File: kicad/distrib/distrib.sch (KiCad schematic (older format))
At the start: 35 parts, among them J1 Conn_01x03_Male, J10 Conn_01x03_Male, J11 Conn_01x03_Male, J12 Conn_01x03_Male, J13 Conn_01x03_Male, J14 Conn_01x03_Male, J15 Conn_01x03_Male, J16 Conn_01x03_Male, J17 Conn_01x03_Male, J18 Conn_01x03_Male, J19 Conn_01x03_Male, J2 Conn_01x03_Male, J20 Conn_01x03_Male, J21 Conn_01x03_Male, J22 Conn_01x03_Male, J23 Conn_01x03_Male, J24 Conn_01x03_Male, J25 Conn_01x03_Male, J26 Conn_01x03_Male, J27 Conn_01x03_Male, J28 Conn_01x03_Male, J29 Conn_01x03_Male, J3 Conn_01x03_Male, J30 Conn_01x03_Male, J31 Screw_Terminal_01x02, J4 Conn_01x03_Male, J5 Conn_01x03_Male, J6 Conn_01x03_Male, J7 Conn_01x03_Male, J8 Conn_01x03_Male, J9 Conn_01x03_Male

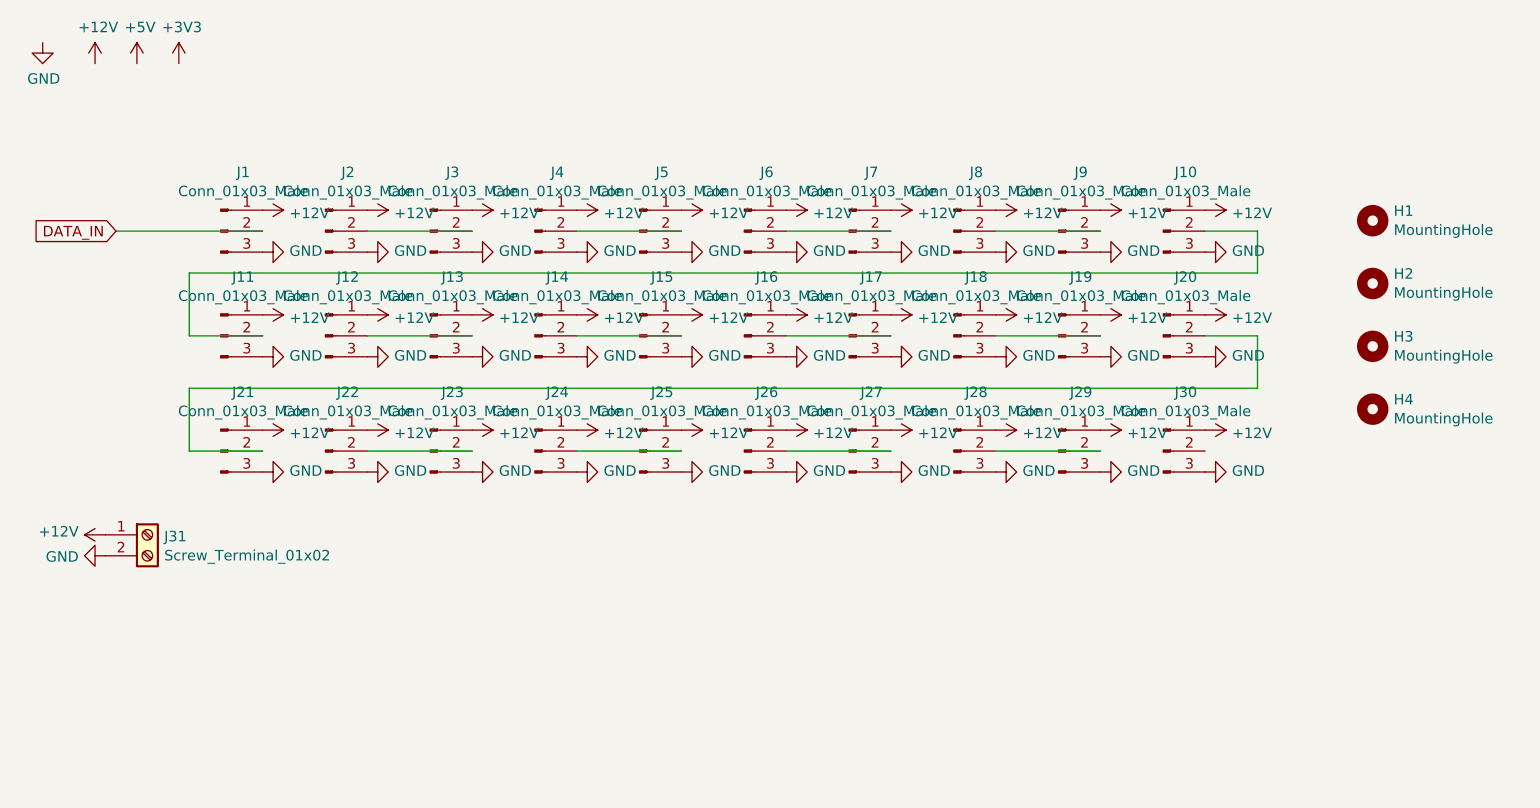
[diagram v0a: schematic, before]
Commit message: breakout
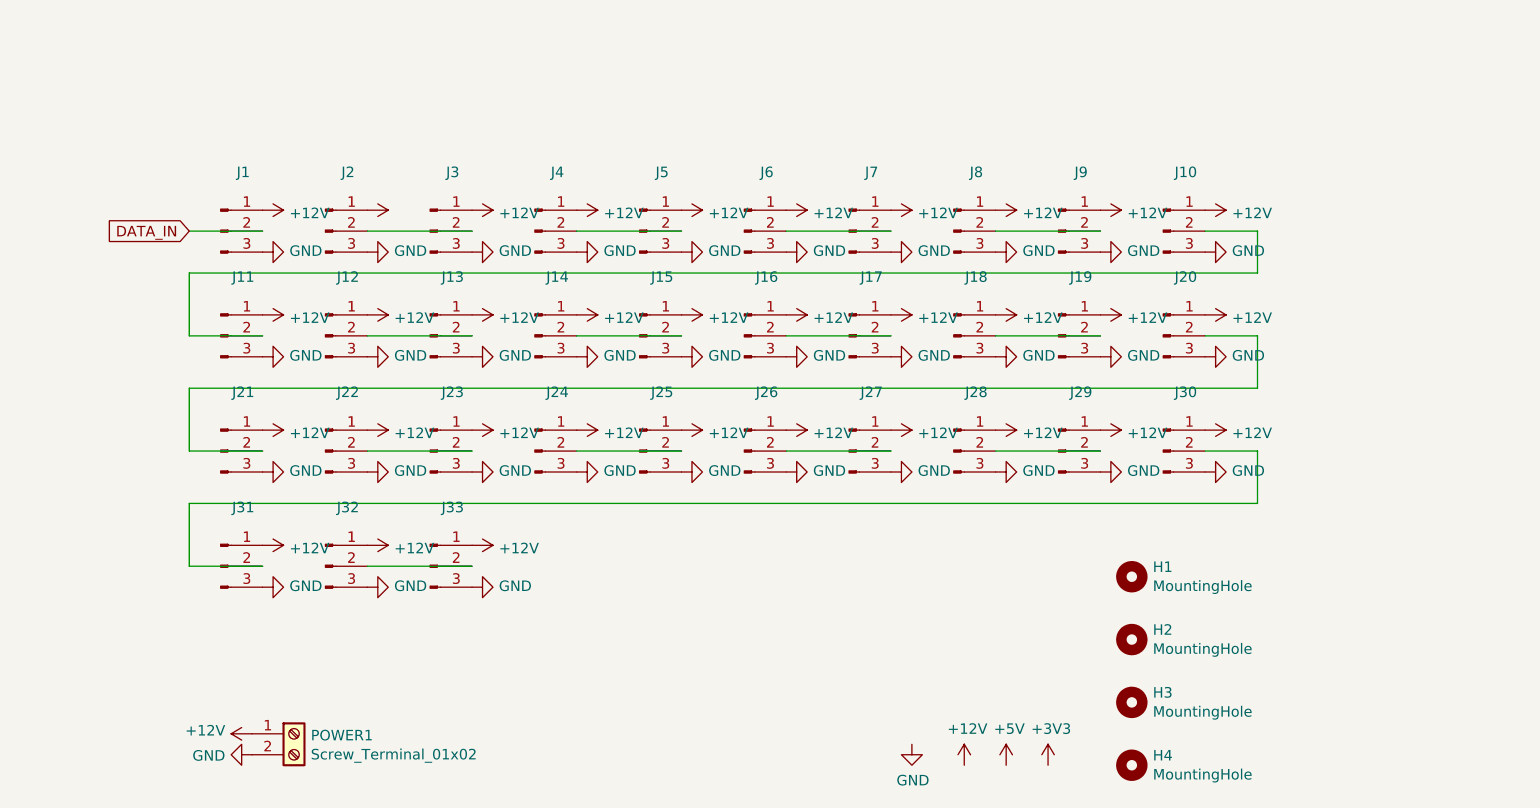
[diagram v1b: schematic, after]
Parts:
- added J31, J32, J33: Conn_01x03_Male, Connectors_Phoenix:PhoenixContact_MCV-G_03x3.81mm_Vertical, symbol Connector:Conn_01x03_Male
- J1, J10, J11, J12, J13, J14, J15, J16, J17, J18, J19, J2, J20, J21, J22, J23, J24, J25, J26, J27, J28, J29, J3, J30, J4, J5, J6, J7, J8, J9: footprint Connectors_Molex:Molex_KK-6410-03_03x2.54mm_Straight -> Connectors_Phoenix:PhoenixContact_MCV-G_03x3.81mm_Vertical
- POWER1: renamed from J31; footprint Connectors_Molex:Molex_KK-6410-02_02x2.54mm_Straight -> Connector_AMASS:AMASS_XT60-F_1x02_P7.20mm_Vertical
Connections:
- net +12V: now also J31.1 (Pin_1), J32.1 (Pin_1), J33.1 (Pin_1)
- net GND: now also J31.3 (Pin_3), J32.3 (Pin_3), J33.3 (Pin_3)
- net at J30.2 (Pin_2): now also J31.2 (Pin_2)
- new net: J32.2 (Pin_2), J33.2 (Pin_2)
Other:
- moved on the sheet: H1, H2, H3, H4, POWER1
